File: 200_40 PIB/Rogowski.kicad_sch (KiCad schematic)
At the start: 8 parts, among them J7 MMCX, U11 OP37

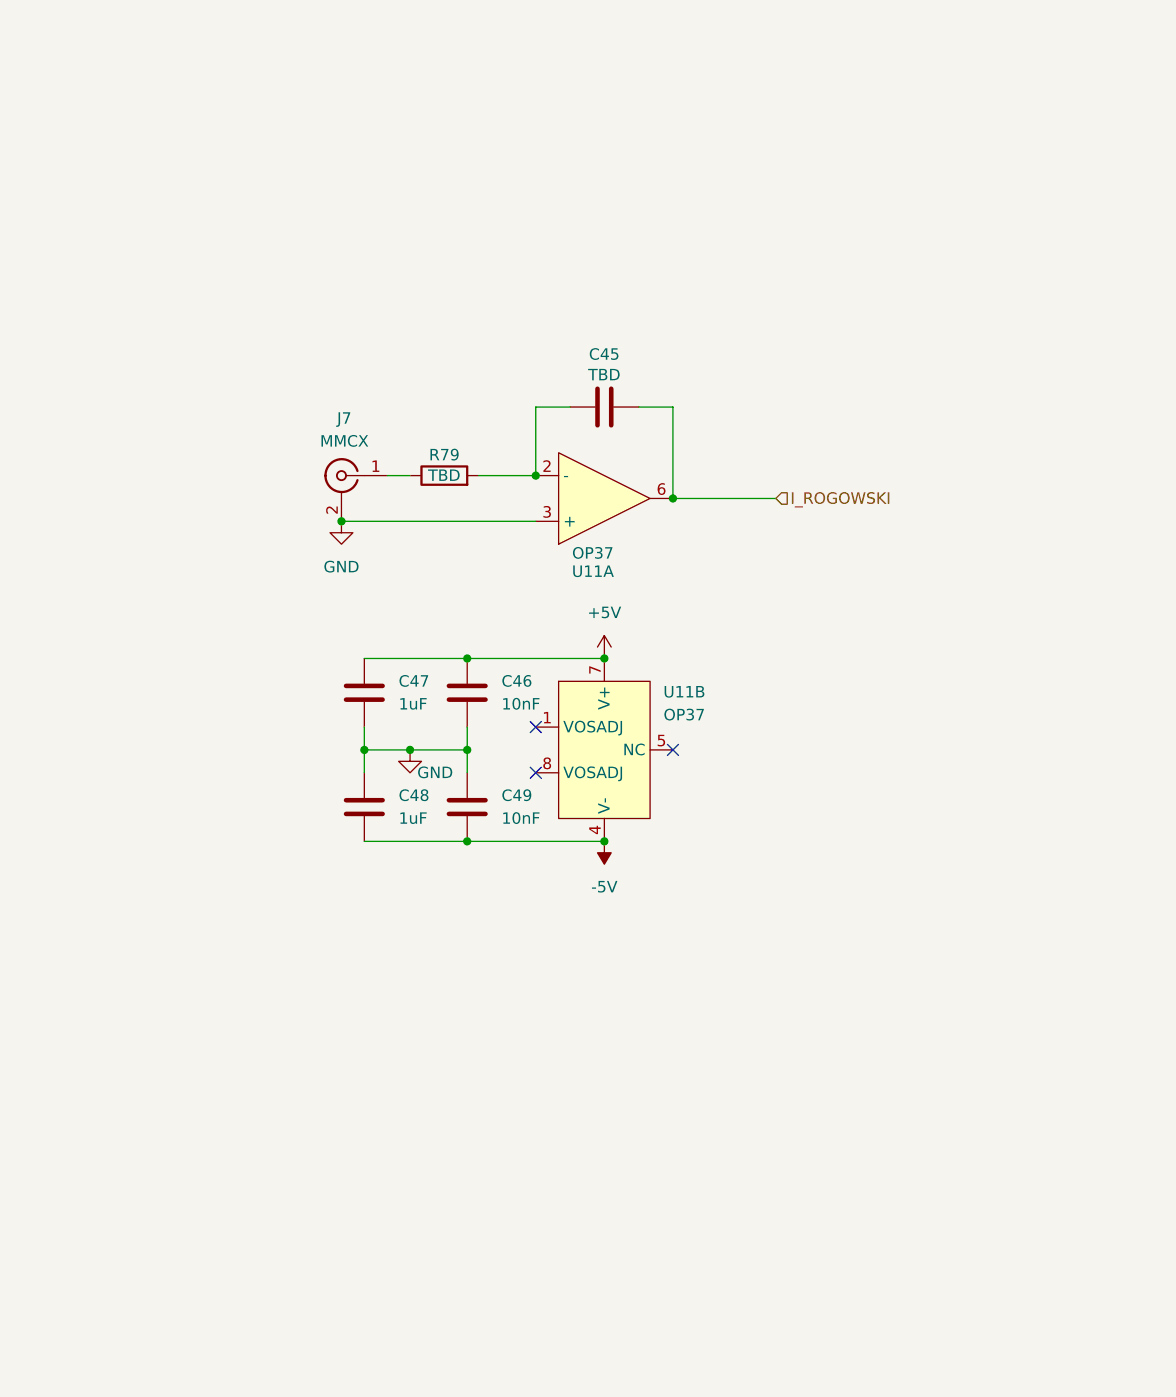
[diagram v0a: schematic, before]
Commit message: clear out claude flagged items
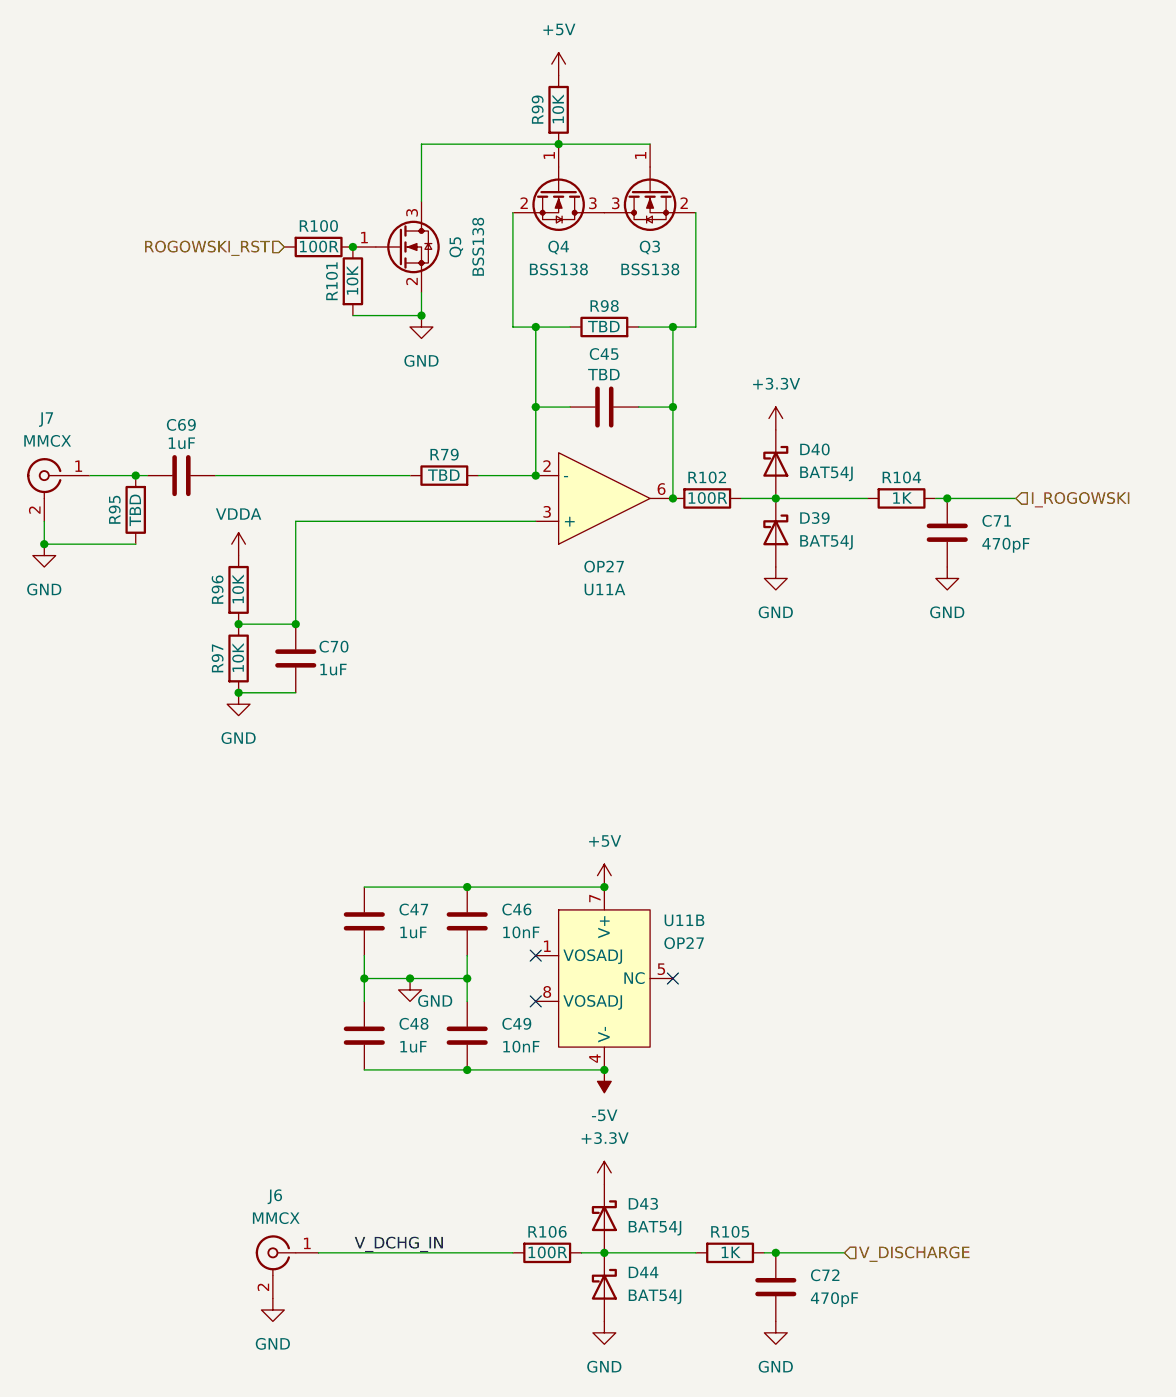
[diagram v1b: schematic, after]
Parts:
- removed U11: OP37, Package_SO:SOIC-8_3.9x4.9mm_P1.27mm, symbol 0_PAY_Symbol_Library:OP37
- added C69, C70: 1uF, Capacitor_SMD:C_0603_1608Metric, symbol Device:C
- added C71, C72: 470pF, Capacitor_SMD:C_0402_1005Metric, symbol Device:C
- added D39, D40, D43, D44: BAT54J, Diode_SMD:D_SOD-323F, symbol Diode:BAT54J
- added J6: MMCX, Connector_Coaxial:MMCX_Molex_73415-1471_Vertical, symbol Connector:Conn_Coaxial
- added Q3, Q4, Q5: BSS138, Package_TO_SOT_SMD:SOT-23, symbol Transistor_FET:BSS138
- added R100, R102, R106: 100R, Resistor_SMD:R_0402_1005Metric, symbol Device:R
- added R101, R96, R97, R99: 10K, Resistor_SMD:R_0402_1005Metric, symbol Device:R
- added R104, R105: 1K, Resistor_SMD:R_0402_1005Metric, symbol Device:R
- added R95, R98: TBD, Resistor_SMD:R_0603_1608Metric, symbol Device:R
- added U11: OP27, Package_SO:SOIC-8_3.9x4.9mm_P1.27mm, symbol 0_PAY_Symbol_Library:OP27
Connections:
- net +5V: now also R99.1, U11.7 (V+)
- net -5V: now also U11.4 (V-)
- net GND: now also C70.2, C71.2, C72.2, D39.2 (A), D44.2 (A), J6.2 (Ext), Q5.2 (S), R101.2, R95.1, R97.2
- net I_ROGOWSKI: now also C71.1, R104.1; no longer C45.2
- net at C45.1, R79.2: now also Q4.2 (S), R98.1, U11.2 (-)
- net at J7.1 (In): now also C69.1, R95.2; no longer R79.1
- new net: C70.1, R96.2, R97.1, U11.3 (+)
- new net: C45.2, Q3.2 (S), R102.2, R98.2, U11.6
- new net: Q5.1 (G), R100.1, R101.1
- new net: D39.1 (K), D40.2 (A), R102.1, R104.2
- new net: D43.2 (A), D44.1 (K), R105.2, R106.1
- new net: C69.2, R79.1
- new net: Q3.1 (G), Q4.1 (G), Q5.3 (D), R99.2
- new net: Q3.3 (D), Q4.3 (D)
- new net +3.3V: D40.1 (K), D43.1 (K)
- new net ROGOWSKI_RST: R100.2
- new net VDDA: R96.1
- new net V_DCHG_IN: J6.1 (In), R106.2
- new net V_DISCHARGE: C72.1, R105.1
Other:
- moved on the sheet: C46, C47, C48, C49, J7
